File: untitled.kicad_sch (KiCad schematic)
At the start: 17 parts, among them CN1 XT30PW-M, CN2 XT30PW-M, SW1 SWITCH_BLACK, SW2 SWITCH_BLACK, U14 XL4005, U15 XC6220B331MR

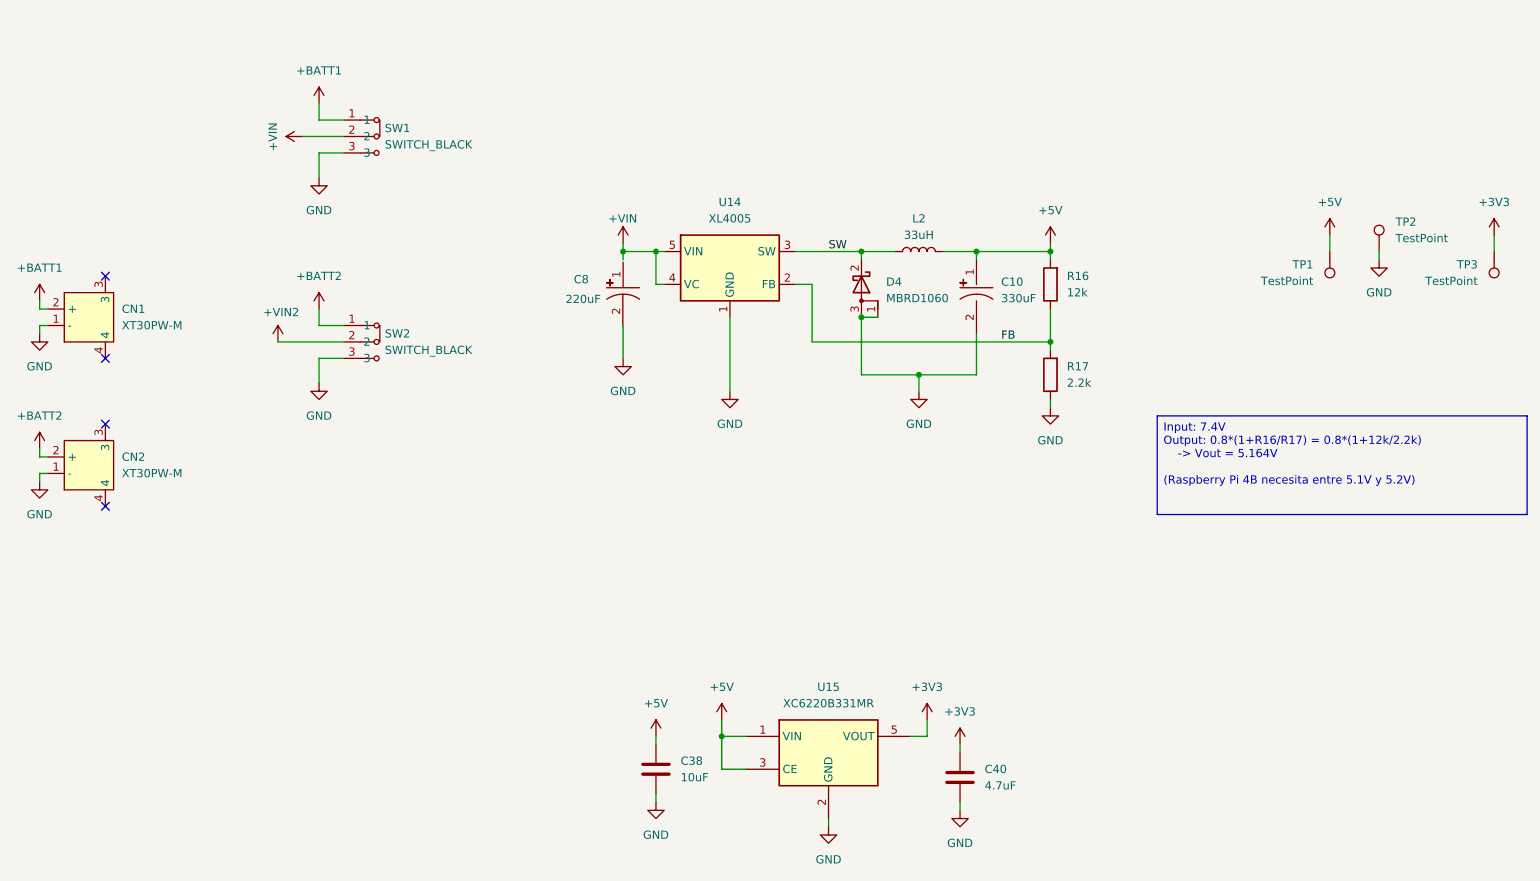
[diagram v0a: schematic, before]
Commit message: BECERRA
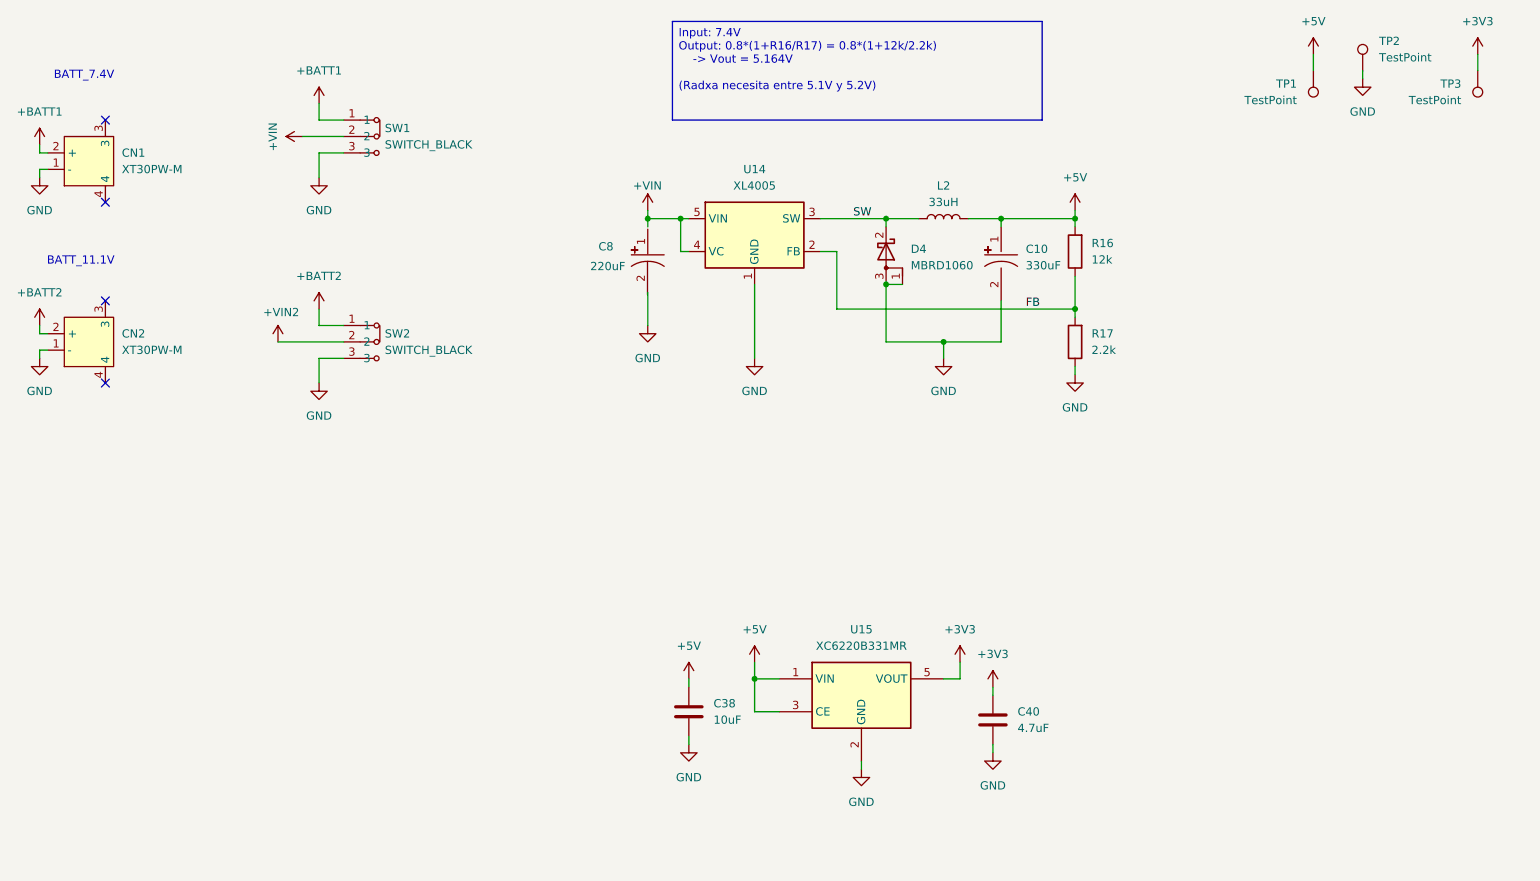
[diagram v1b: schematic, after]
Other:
- note added: "BATT_11.1V"
- note added: "BATT_7.4V"
- moved on the sheet: C10, C38, C40, C8, CN1, CN2, D4, L2, R16, R17, TP1, TP2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
